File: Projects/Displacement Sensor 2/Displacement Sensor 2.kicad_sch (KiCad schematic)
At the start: 11 parts, among them U1 TJA1050DRG, U2 MCP2515-I, X1 ${ALTIUM_VALUE}

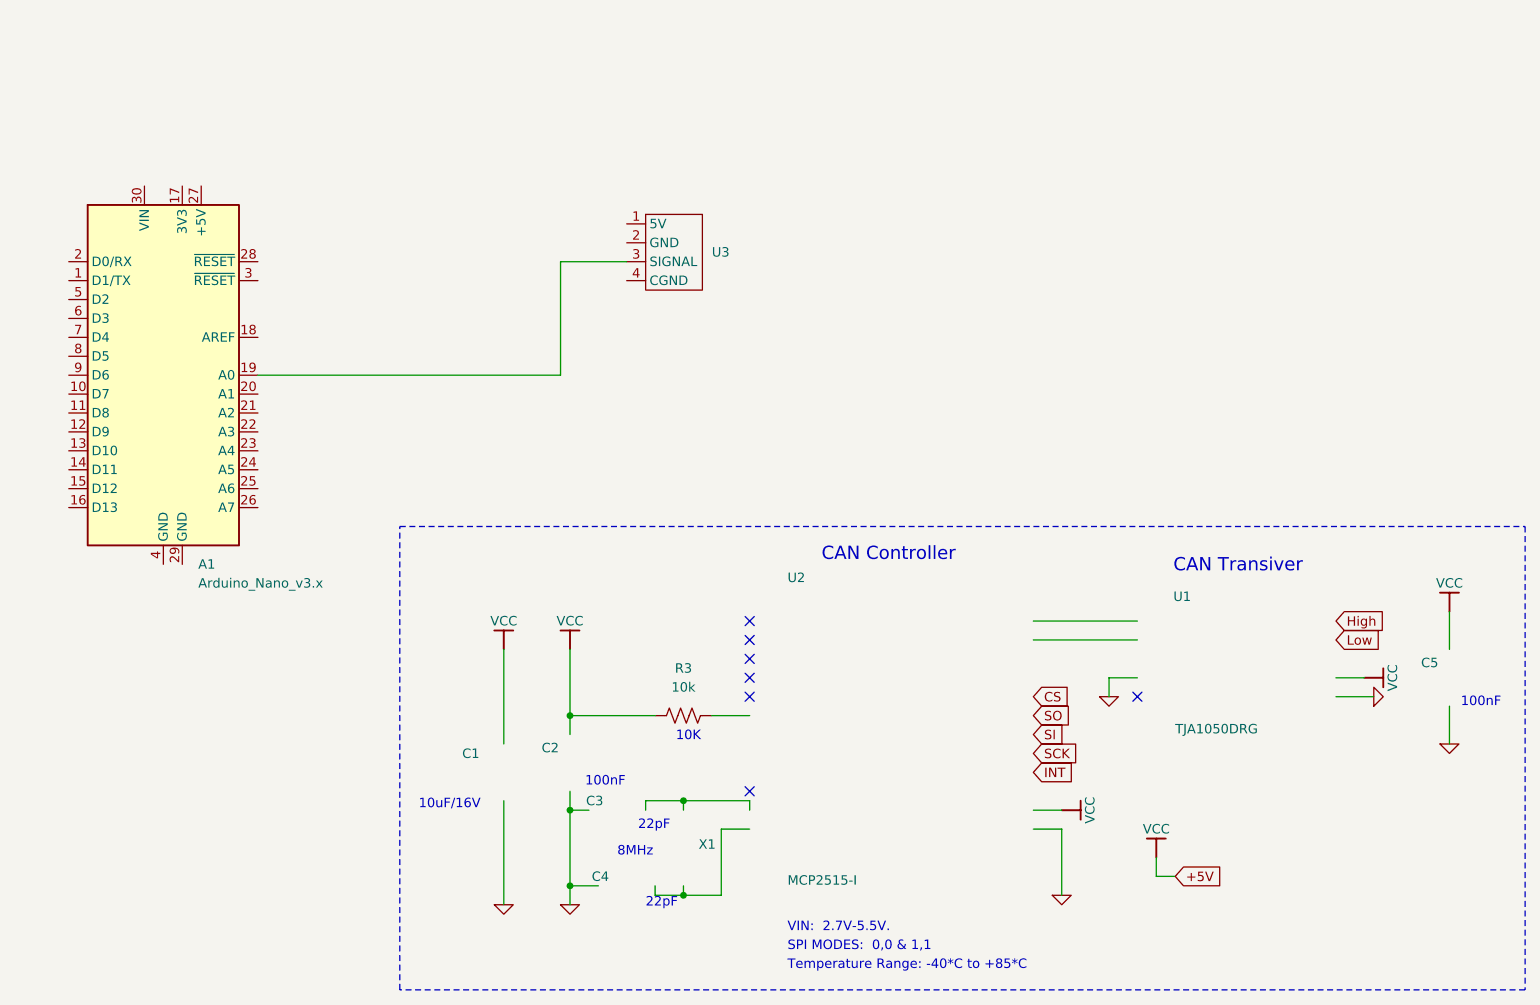
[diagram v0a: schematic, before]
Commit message: Finished displacement schem
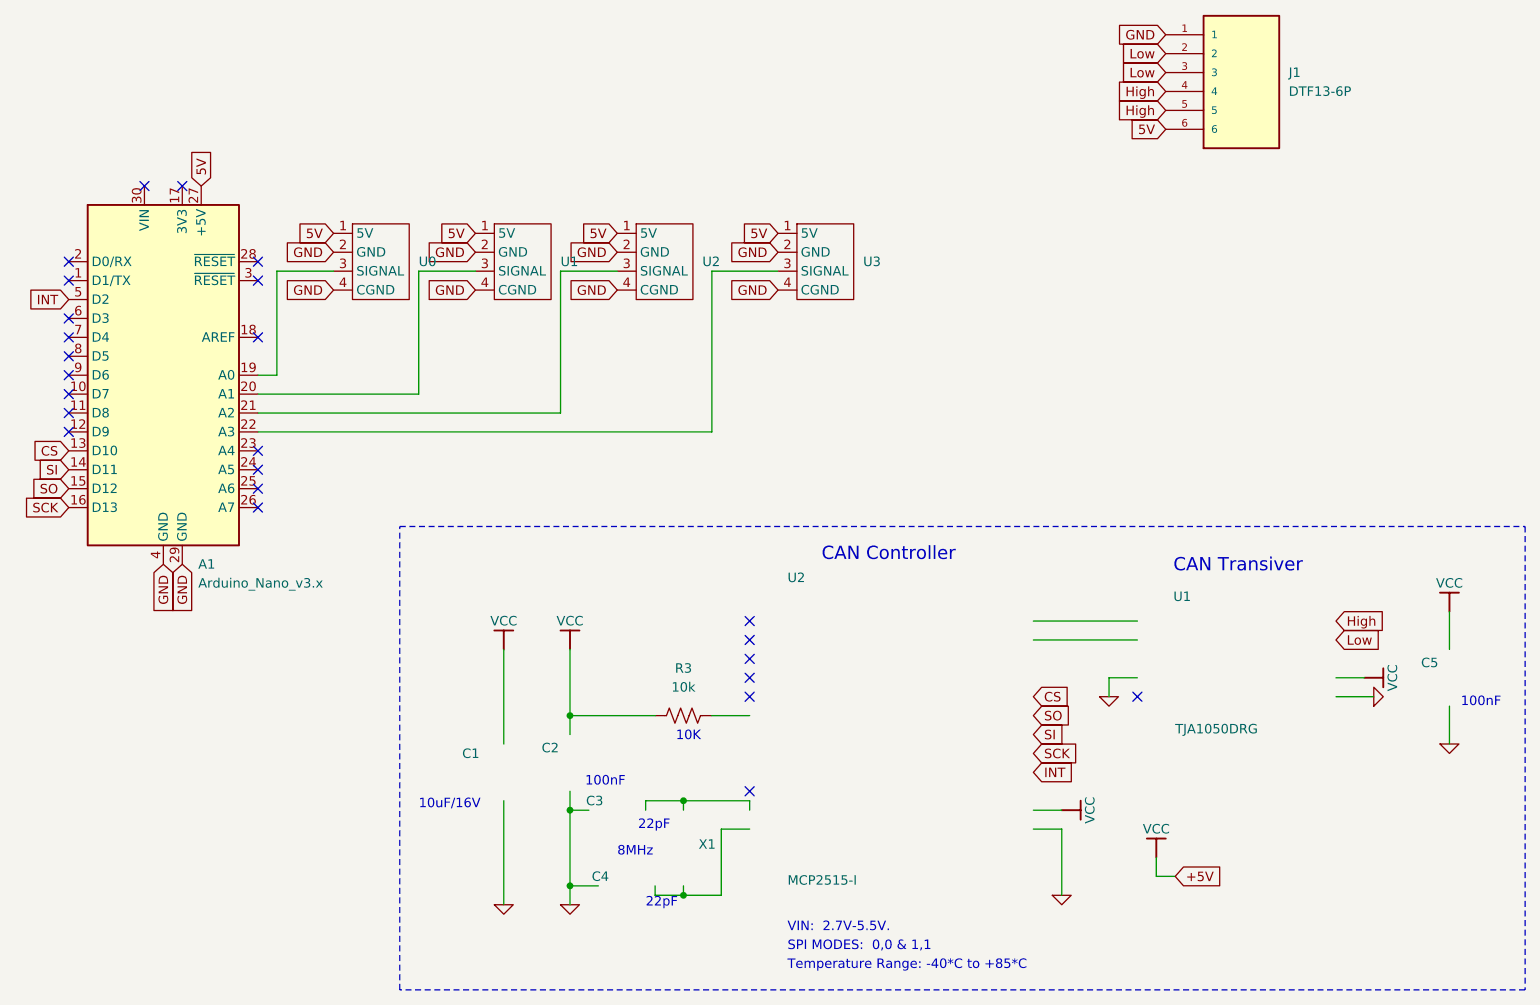
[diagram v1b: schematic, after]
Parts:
- added J1: DTF13-6P, DTF13-6P:TE_DTF13-6P, symbol DTF13-6P:DTF13-6P
- added unit 1 of U1
- added unit 1 of U2
- added U3: (no value), symbol Displacement Pins:Displacement_pins
- renumbered U3 to U0
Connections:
- net CS: now also A1.13 (D10)
- net High: now also J1.4, J1.5
- net INT: now also A1.5 (D2)
- net Low: now also J1.2, J1.3
- net SCK: now also A1.16 (D13)
- net SI: now also A1.14 (D11)
- net SO: now also A1.15 (D12)
- net 5V: now reaches U0.1 (5V)
- net 5V: now also A1.27 (+5V), J1.6, U1.1 (5V), U2.1 (5V), U3.1 (5V)
- net GND: now reaches U0.2 (GND)
- net GND: now also A1.29 (GND), A1.4 (GND), U0.4 (CGND), J1.1, U1.2 (GND), U1.4 (CGND), U2.2 (GND), U2.4 (CGND), U3.2 (GND), U3.4 (CGND)
- net at A1.20 (A1): now also U1.3 (SIGNAL)
- net at A1.21 (A2): now also U2.3 (SIGNAL)
- net at A1.22 (A3): now also U3.3 (SIGNAL)
- no-connect marks 7 -> 25
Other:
- moved on the sheet: U0
